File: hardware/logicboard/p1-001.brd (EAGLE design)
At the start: 91 x 57 mm, 36 parts, among them J7 DIN5, K1 G5V1, K1B G5V1, K1C G5V1, T1 2SC1815, T1B 2SC1815, T1C 2SC1815

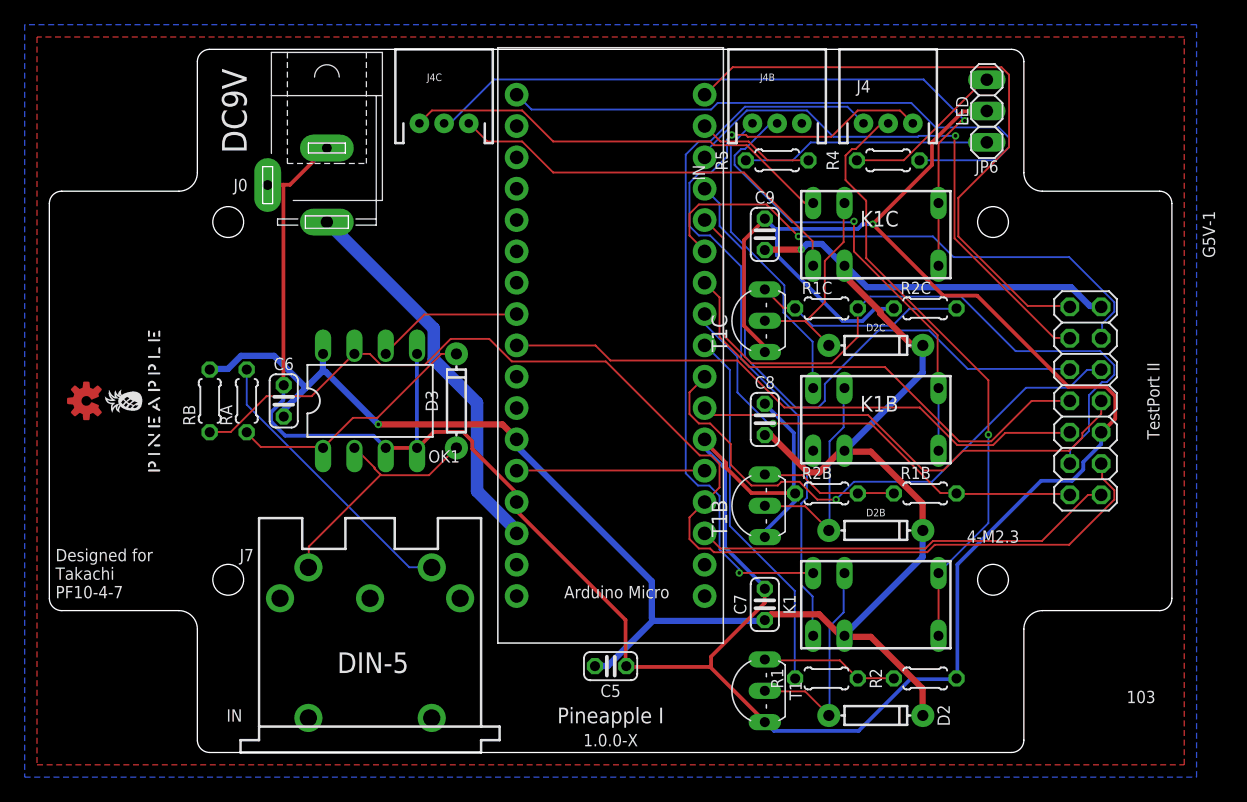
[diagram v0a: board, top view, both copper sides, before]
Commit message: Autorouted.
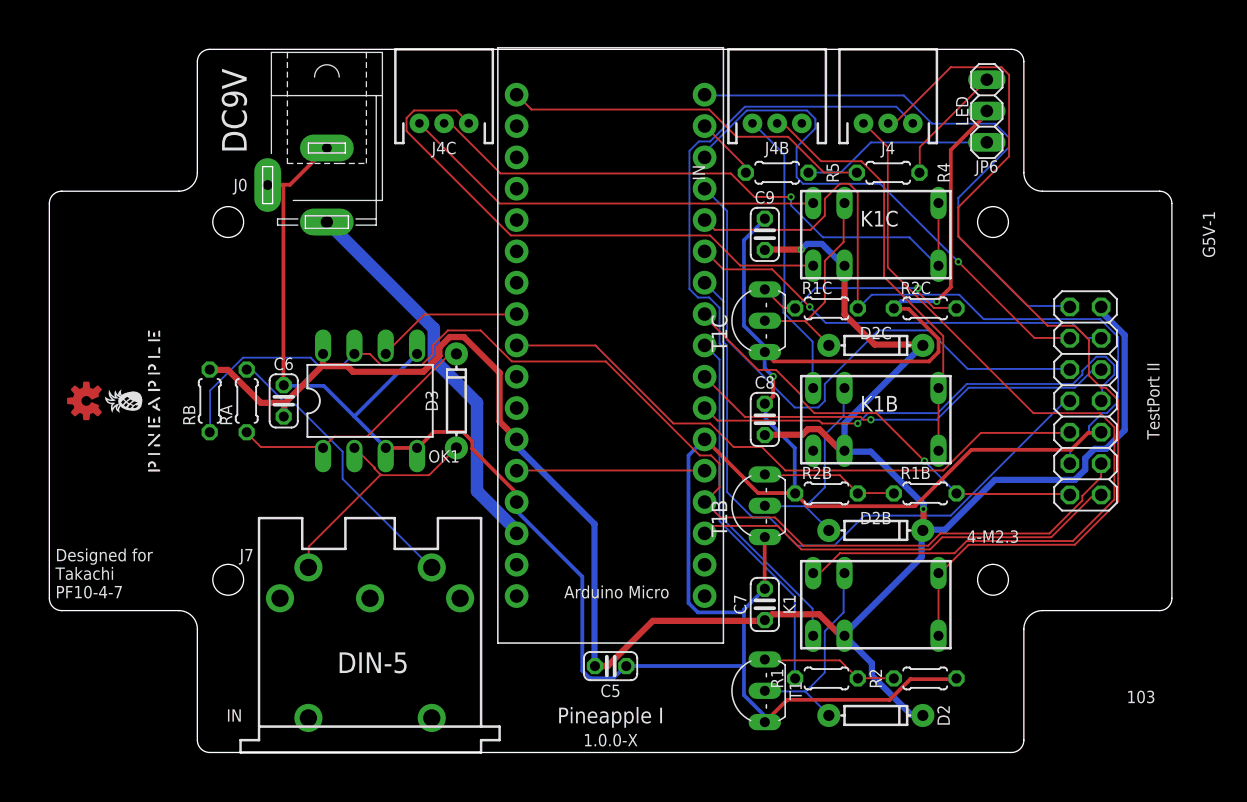
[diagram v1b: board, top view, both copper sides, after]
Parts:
- moved R4 1.00 mm to (68.0, 47.0), turned to 180 degrees
- moved R5 1.00 mm to (59.0, 47.0), turned to 180 degrees
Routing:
- net RLYOUT2: track 49.9 -> 77.2 mm, vias 1 -> 0
- net LED0: track 50.3 -> 30.2 mm
- net GND: track 255.3 -> 239.3 mm, vias 1 -> 2
- net DTCT0: track 38.2 -> 52.2 mm
- net VCC: track 166.3 -> 180.1 mm
- net RLYOUT3C: track 33.9 -> 44.3 mm
- net RLYOUT1: track 58.8 -> 69.0 mm, vias 1 -> 0
- net SCL: track 45.4 -> 35.3 mm
- net D7GATE: track 45.0 -> 35.1 mm
- net RLYOUT2C: track 57.9 -> 50.3 mm
- net DTCT3: track 52.1 -> 47.2 mm
- net LED1A: track 20.1 -> 15.5 mm
- net LED1: track 9.56 -> 5.21 mm
- net RLYOUT2B: track 38.4 -> 34.5 mm, vias 1 -> 0
- net LED0A: track 13.3 -> 9.80 mm
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- removed copper zone on layer 1, net GND
- removed copper zone on layer 16, net GND
